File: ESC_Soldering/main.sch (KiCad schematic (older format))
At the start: 11 parts, among them P1 CONN_02X03, P2 CONN_01X03, P3 CONN_01X03, P4 CONN_01X02, P5 CONN_02X05, U1 PCA9698, U2 ADS7828

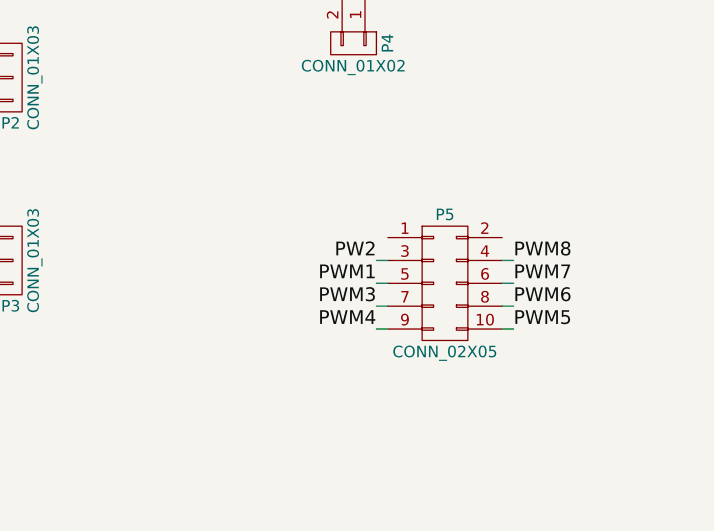
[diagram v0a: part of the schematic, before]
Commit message: test
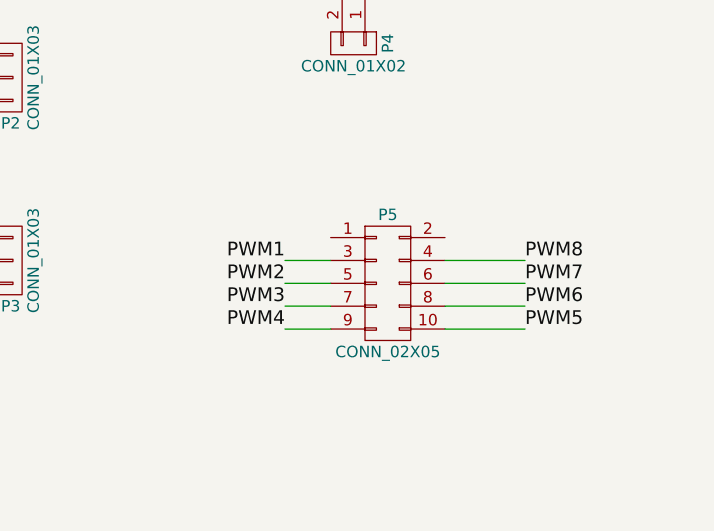
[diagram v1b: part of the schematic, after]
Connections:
- net PW2 is gone; now on net PWM1: P5.3 (P3)
- net PWM1: no longer P5.5 (P5)
- new net PWM2: P5.5 (P5)
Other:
- moved on the sheet: P5
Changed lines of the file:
@@
 L CONN_02X05 P5
 U 1 1 584FCE49
-P 9500 5350
-F 0 "P5" H 9500 5650 50  0000 C CNN
-F 1 "CONN_02X05" H 9500 5050 50  0000 C CNN
-F 2 "Pin_Headers:Pin_Header_Straight_2x05" H 9500 4150 50  0001 C CNN
-F 3 "" H 9500 4150 50  0000 C CNN
-	1    9500 5350
+P 9250 5350
+F 0 "P5" H 9250 5650 50  0000 C CNN
+F 1 "CONN_02X05" H 9250 5050 50  0000 C CNN
+F 2 "Pin_Headers:Pin_Header_Straight_2x05" H 9250 4150 50  0001 C CNN
+F 3 "" H 9250 4150 50  0000 C CNN
+	1    9250 5350
 	1    0    0    -1
 $EndComp
-Text Label 9800 5550 0    60   ~ 0
+Text Label 9850 5550 0    60   ~ 0
 PWM5
-Text Label 9800 5450 0    60   ~ 0
+Text Label 9850 5450 0    60   ~ 0
 PWM6
-Text Label 9800 5350 0    60   ~ 0
+Text Label 9850 5350 0    60   ~ 0
 PWM7
-Text Label 9800 5250 0    60   ~ 0
+Text Label 9850 5250 0    60   ~ 0
 PWM8
-Text Label 9200 5550 2    60   ~ 0
+Text Label 8800 5550 2    60   ~ 0
 PWM4
-Text Label 9200 5450 2    60   ~ 0
+Text Label 8800 5450 2    60   ~ 0
 PWM3
-Text Label 9200 5350 2    60   ~ 0
+Text Label 8800 5250 2    60   ~ 0
 PWM1
 Wire Wire Line
-	9800 5250 9750 5250
+	9850 5250 9500 5250
 Wire Wire Line
-	9750 5350 9800 5350
+	9500 5350 9850 5350
 Wire Wire Line
-	9800 5450 9750 5450
+	9850 5450 9500 5450
 Wire Wire Line
-	9750 5550 9800 5550
+	9500 5550 9850 5550
+Text Label 8800 5350 2    60   ~ 0
+PWM2
 Wire Wire Line
-	9250 5550 9200 5550
+	8800 5550 9000 5550
 Wire Wire Line
-	9200 5450 9250 5450
+	9000 5250 8800 5250
 Wire Wire Line
-	9200 5250 9250 5250
+	8800 5450 9000 5450
 Wire Wire Line
-	9250 5350 9200 5350
-Text Label 9200 5250 2    60   ~ 0
-PW2
+	8800 5350 9000 5350
 $EndSCHEMATC
